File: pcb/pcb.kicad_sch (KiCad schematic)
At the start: 54 parts, among them J1 Conn_01x20, J2 Conn_01x20, J3 Battery, J4 Ultrasonic eyes, M1 Motor_L, M2 Motor_R, Q1 AO3401A, U1 QRE1113GR, U10 DRV8220SDG, U2 QRE1113GR, U3 QRE1113GR, U4 QRE1113GR, U5 QRE1113GR, U6 QRE1113GR, U7 QRE1113GR, U8 QRE1113GR, U9 DRV8220SDG

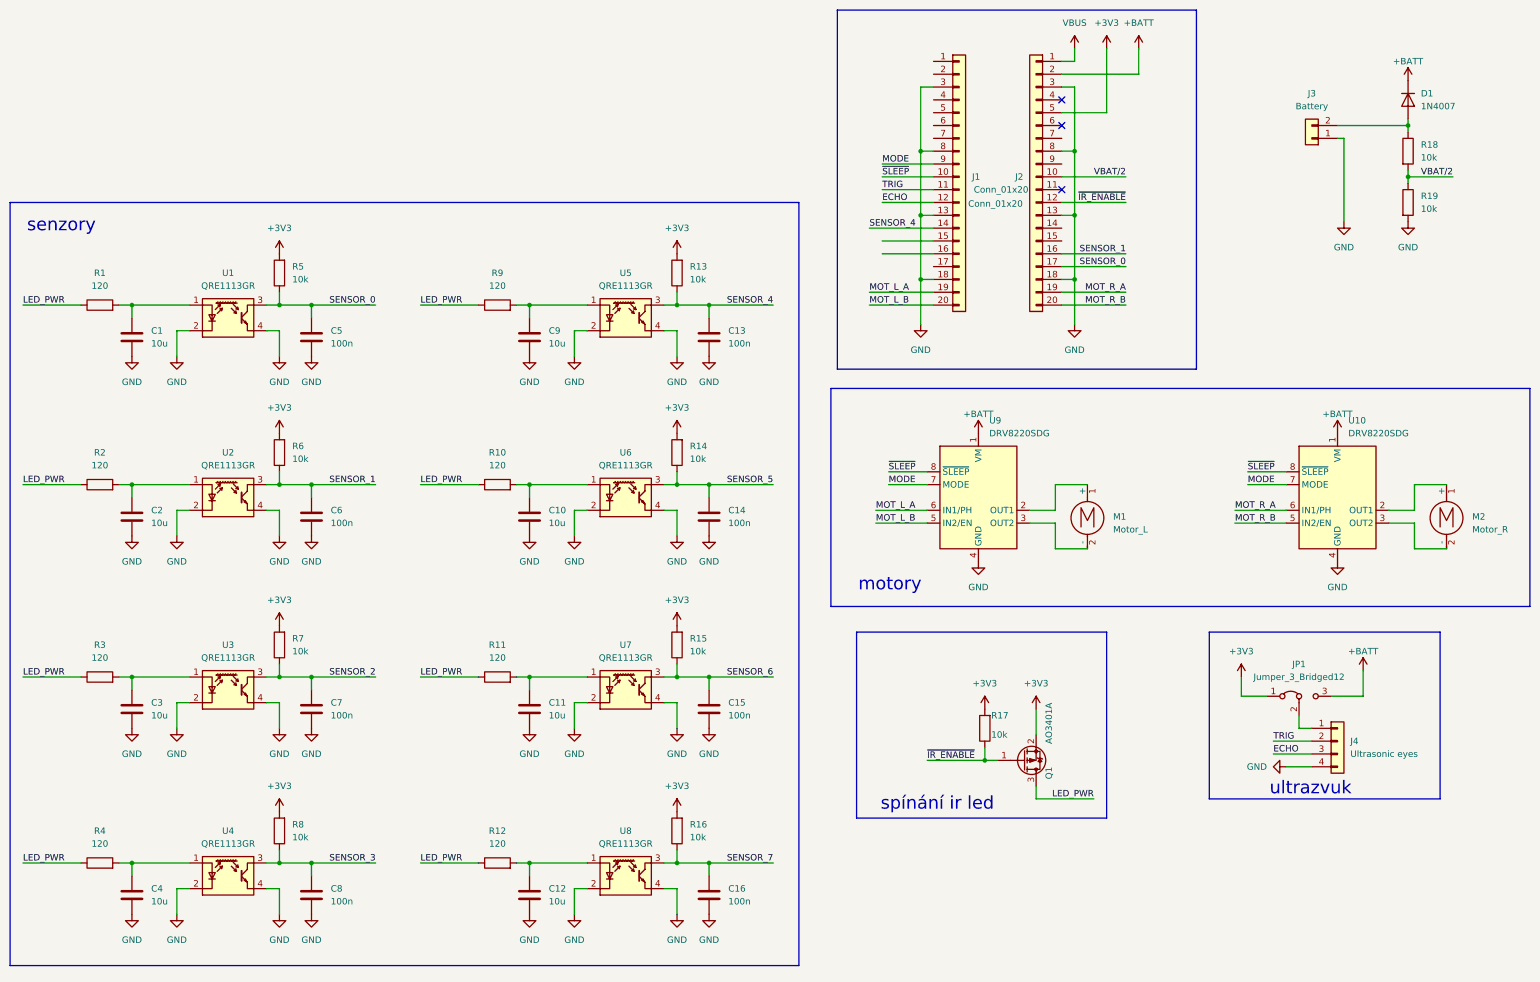
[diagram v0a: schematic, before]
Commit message: Úklid schématu
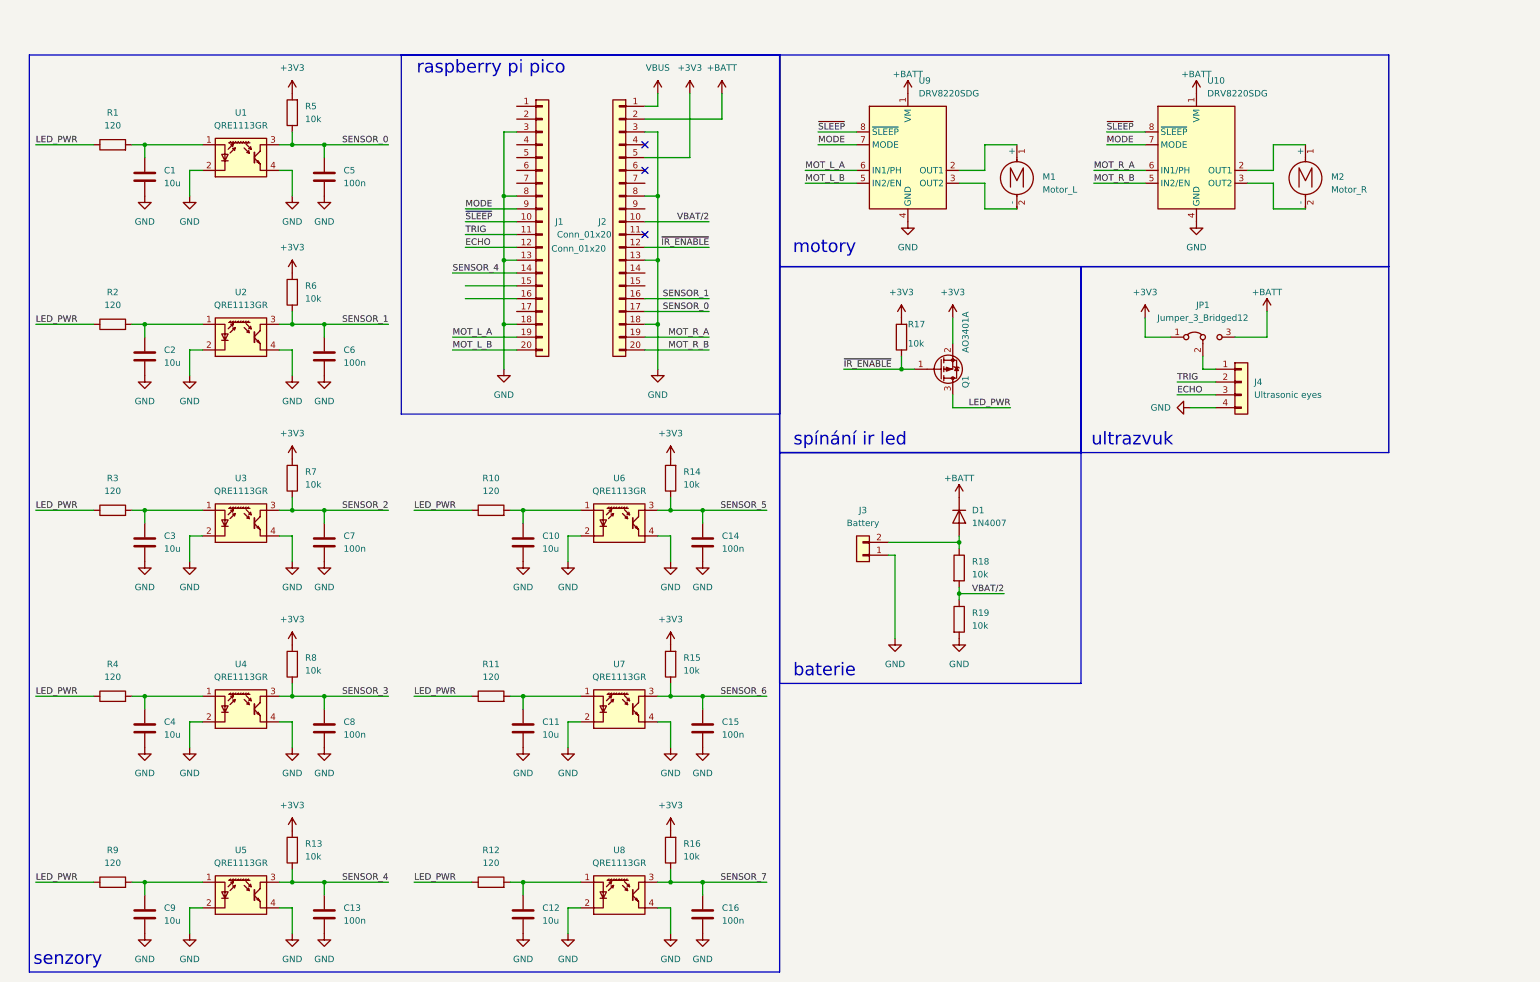
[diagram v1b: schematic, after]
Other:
- note added: "baterie"
- note added: "raspberry pi pico"
- moved on the sheet: C1, C10, C11, C12, C13, C14, C15, C16, C2, C3, C4, C5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
